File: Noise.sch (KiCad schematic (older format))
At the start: 13 parts, among them Q1 Q_NPN_BCE, Q2 2N3904

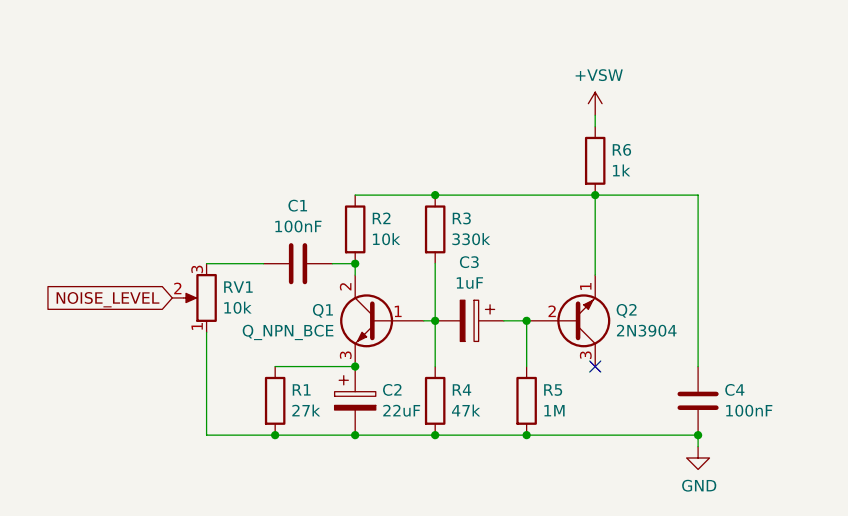
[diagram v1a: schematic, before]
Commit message: Create pcb and other updates
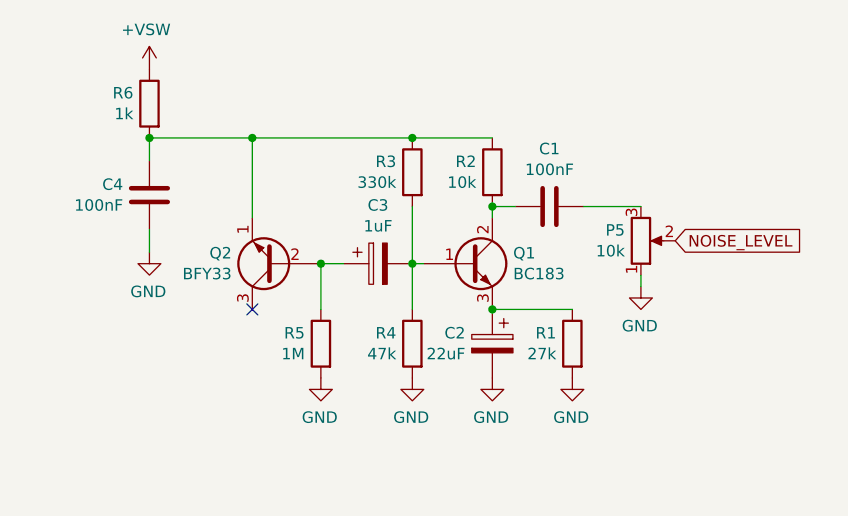
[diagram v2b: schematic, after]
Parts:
- C1, C4: footprint (none) -> Capacitor_THT:C_Disc_D5.0mm_W2.5mm_P5.00mm
- C2, C3: footprint (none) -> Capacitor_THT:CP_Radial_D6.3mm_P2.50mm
- P5: renamed from RV1; footprint (none) -> Connector_PinSocket_2.54mm:PinSocket_1x03_P2.54mm_Vertical
- Q1: value Q_NPN_BCE -> BC183; footprint (none) -> Package_TO_SOT_THT:TO-92L_Inline_Wide
- Q2: value 2N3904 -> BFY33; footprint Package_TO_SOT_THT:TO-92_Inline -> Package_TO_SOT_THT:TO-92L_Inline_Wide
- R1, R2, R3, R4, R5, R6: footprint (none) -> Resistor_THT:R_Axial_DIN0207_L6.3mm_D2.5mm_P10.16mm_Horizontal
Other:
- moved on the sheet: C1, C2, C3, C4, P5, Q1, Q2, R1, R2, R3, R4, R5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
